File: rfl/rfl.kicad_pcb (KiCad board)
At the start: 4 copper layers, 20 x 30 mm, 37 parts, among them J1 636101111001, J2 Conn_01x09, J801 629722000214, J802 swd, U1 SX1281, U2 STM32G0B1KETxN, U3 TPS7A19, U801 USBLC6-2SC6, Y1 52MHz

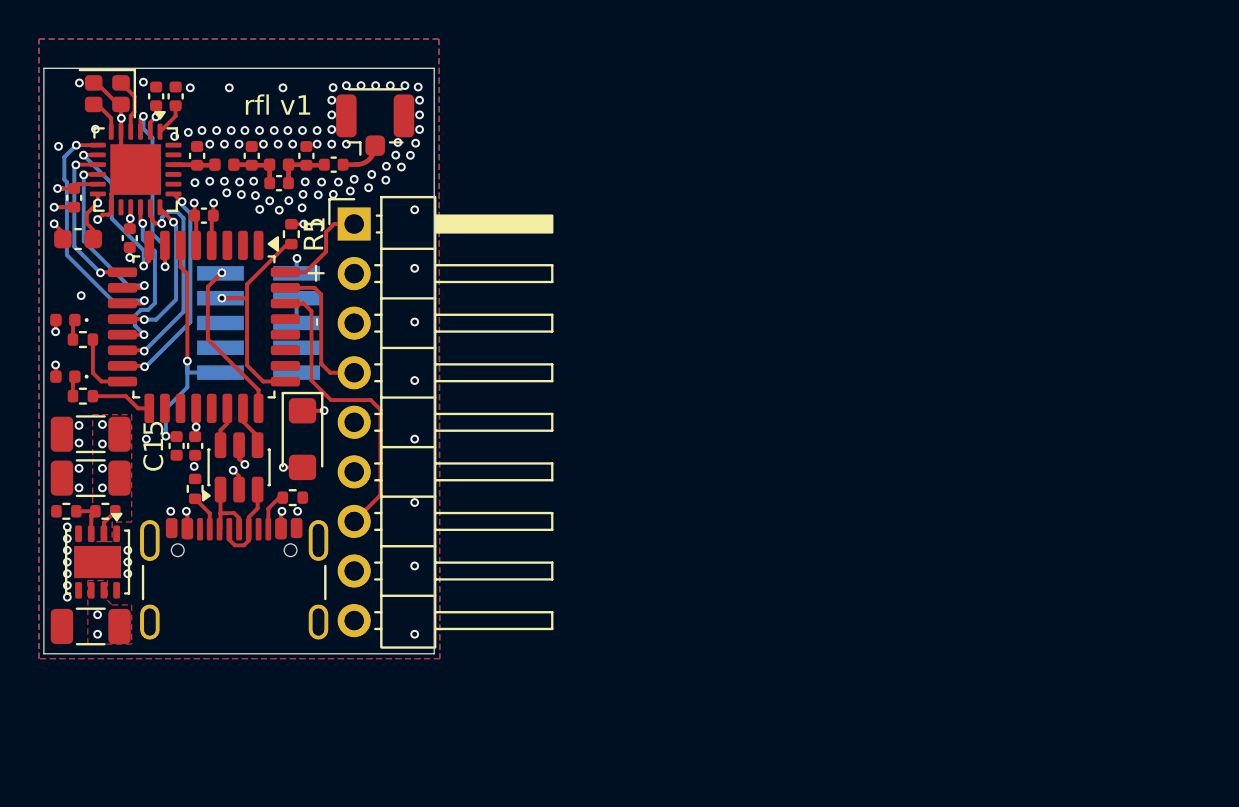
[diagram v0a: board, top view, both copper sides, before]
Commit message: v2 with rf switch wip
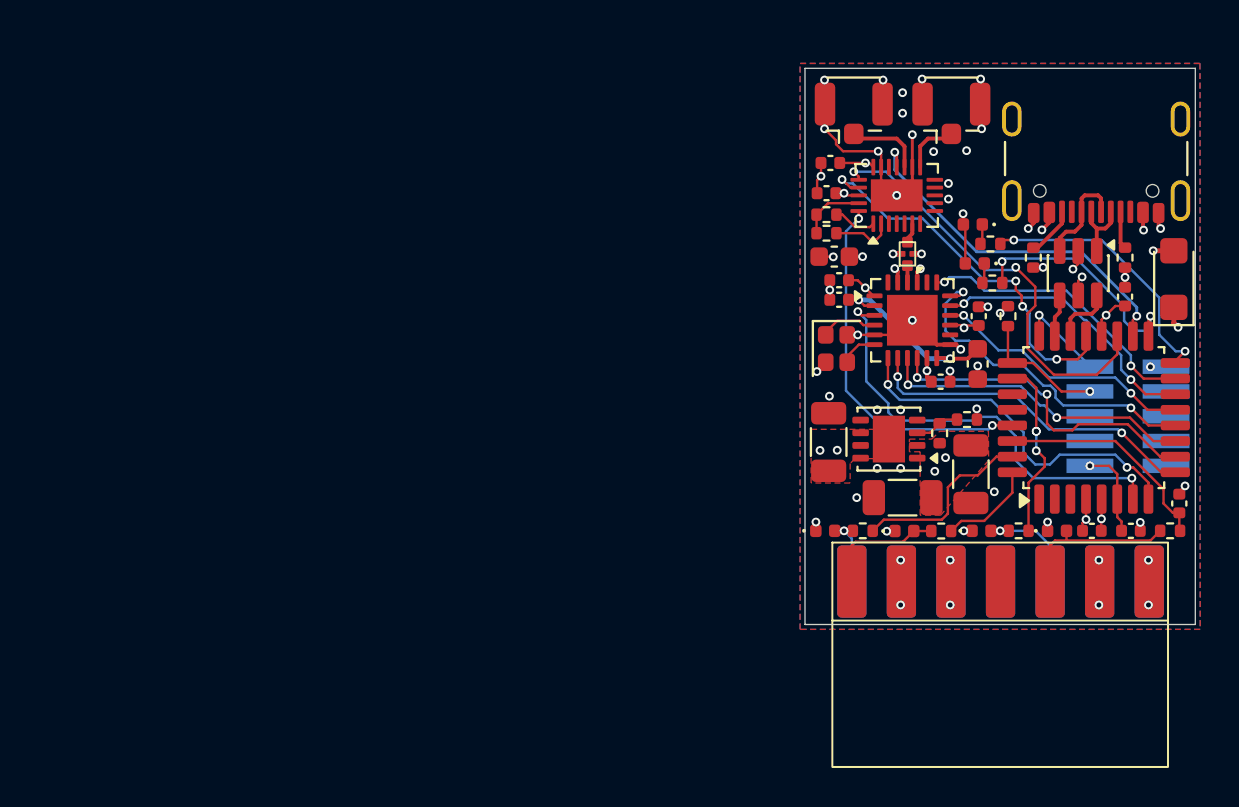
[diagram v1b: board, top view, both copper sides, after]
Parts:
- removed C11, C12: C, Capacitor_SMD:C_0402_1005Metric
- removed L3, L4: L, Inductor_SMD:L_0402_1005Metric
- added C8: C, Capacitor_SMD:C_0603_1608Metric, F.Cu at (210.5, 77.7)
- added D3: D_TVS, Diode_SMD:D_0402_1005Metric, F.Cu at (218.0, 91.7)
- added D4: D_TVS, Diode_SMD:D_0402_1005Metric, F.Cu at (221.9, 91.7)
- added D5: D_TVS, Diode_SMD:D_0402_1005Metric, F.Cu at (210.0, 91.7)
- added D6: D_TVS, Diode_SMD:D_0402_1005Metric, F.Cu at (214.1, 91.7)
- added FL1: 2450FM07D0034001T, rfl-lib-fp:2450FM07D0034001T, F.Cu at (214.2, 77.5)
- added J3: 636101111001, Connector_Coaxial:U.FL_Hirose_U.FL-R-SMT-1_Vertical, F.Cu at (211.5, 69.8)
- added R10: R, Resistor_SMD:R_0402_1005Metric, F.Cu at (227.7, 91.7)
- added R11: R, Resistor_SMD:R_0402_1005Metric, F.Cu at (219.9, 91.7)
- added R6: R, Resistor_SMD:R_0402_1005Metric, F.Cu at (210.1, 75.5)
- added R7: R, Resistor_SMD:R_0402_1005Metric, F.Cu at (210.1, 76.5)
- added R8: R, Resistor_SMD:R_0402_1005Metric, F.Cu at (216.0, 91.7)
- added R9: R, Resistor_SMD:R_0402_1005Metric, F.Cu at (212.0, 91.7)
- added U4: SE2431L, Package_DFN_QFN:QFN-24-1EP_3x4mm_P0.4mm_EP1.65x2.65mm, F.Cu at (213.7, 74.5)
- J2: value Conn_01x09 -> Conn_01x14; footprint Connector_PinHeader_2.54mm:PinHeader_1x09_P2.54mm_Horizontal -> rfl-lib-fp:PinHeader_2x07_P2.54mm_Edge
- moved J801 50.1 mm to (223.9, 71.7), turned to 180 degrees
- moved R802 49.1 mm to (225.4, 77.7), turned to 90 degrees
- moved C15 49.1 mm to (225.7, 91.7), turned to 180 degrees
- moved C10 48.1 mm to (228.2, 90.3), turned to -90 degrees
- moved C14 47.4 mm to (225.4, 79.7), turned to -90 degrees
- moved D2 47.0 mm to (217.7, 78.0)
- moved R4 47.0 mm to (218.6, 79.0)
- moved D1 46.8 mm to (217.6, 76.0)
- moved R3 46.8 mm to (218.5, 77.0)
- moved C1 46.5 mm to (217.8, 83.2), turned to -90 degrees
- moved R2 46.4 mm to (217.3, 86.0), turned to 0 degrees
- moved C13 46.2 mm to (223.7, 91.7), turned to 180 degrees
- moved U2 45.8 mm to (223.8, 85.9), turned to 90 degrees
- moved D101 45.4 mm to (227.9, 78.8), turned to 90 degrees
- moved C5 45.4 mm to (215.9, 84.1), turned to 180 degrees
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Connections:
- C10 pad 1: Net-(C10-Pad1) -> GND
- C10 pad 2: GND -> /d3
- C6 pad 1: Net-(U1-RFIO) -> GND
- C6 pad 2: GND -> +3.3V
- C7 pad 1: Net-(C11-Pad1) -> +3.3V
- J2 pad 1: /d1 -> Net-(D6-A2)
- J2 pad 2: VDD -> Net-(D5-A2)
- J2 pad 3: GND -> VDD
- J2 pad 4: /d2 -> VDD
- J2 pad 5: VDD -> GND
- J2 pad 7: /d3 -> unconnected-(J2-Pin_7-Pad7)
- J2 pad 8: VDD -> unconnected-(J2-Pin_8-Pad8)
- J2 pad 9: GND -> Net-(D4-A2)
- U1 pad 22: Net-(U1-RFIO) -> Net-(FL1-IN)
- U2 pad 11: /busy -> /dio2
- U2 pad 18: unconnected-(U2-PA8-Pad18) -> /antsel
- U2 pad 19: unconnected-(U2-PA9/UCPD1_DBCC1-Pad19) -> /csd
- U2 pad 21: unconnected-(U2-PA10/UCPD1_DBCC2-Pad21) -> /cps
- U2 pad 26: unconnected-(U2-PD0-Pad26) -> /d4
- U2 pad 29: unconnected-(U2-PD3-Pad29) -> /ctx
- U2 pad 8: /dio1 -> /busy
- U2 pad 9: /dio2 -> /dio1
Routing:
- net /csd: track 0.00 -> 22.2 mm, vias 0 -> 2
- net /cps: track 0.00 -> 19.7 mm, vias 0 -> 4
- net /ctx: track 0.00 -> 18.9 mm, vias 0 -> 2
- net /antsel: track 0.00 -> 18.6 mm, vias 0 -> 2
- net GND: track 16.2 -> 33.4 mm, vias 104 -> 53
- net /sx_nreset: track 10.1 -> 22.6 mm
- net Net-(U2-PB1): track 3.41 -> 13.8 mm, vias 0 -> 2
- net /d4: track 0.00 -> 9.30 mm, vias 0 -> 3
- net Net-(U2-PB15): track 3.15 -> 12.4 mm, vias 0 -> 2
- net /sck: track 8.25 -> 17.3 mm
- net /dio1: track 8.87 -> 17.5 mm
- net /nreset: track 13.2 -> 4.58 mm, vias 2 -> 1
- net Net-(D4-A2): track 0.00 -> 8.31 mm
- net /dio2: track 8.38 -> 16.3 mm
- net /dio3: track 9.35 -> 17.0 mm
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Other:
- board size 20 x 30 mm -> 20 x 28.5 mm
- board text added: "s"
- board text removed: "1"
- board text removed: "rfl v1"
